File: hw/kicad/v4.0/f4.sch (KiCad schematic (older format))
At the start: 31 parts, among them P1 USB_OTG, U1 USBLC6-4SC6, U26 STM32F405VG, Y2 8M

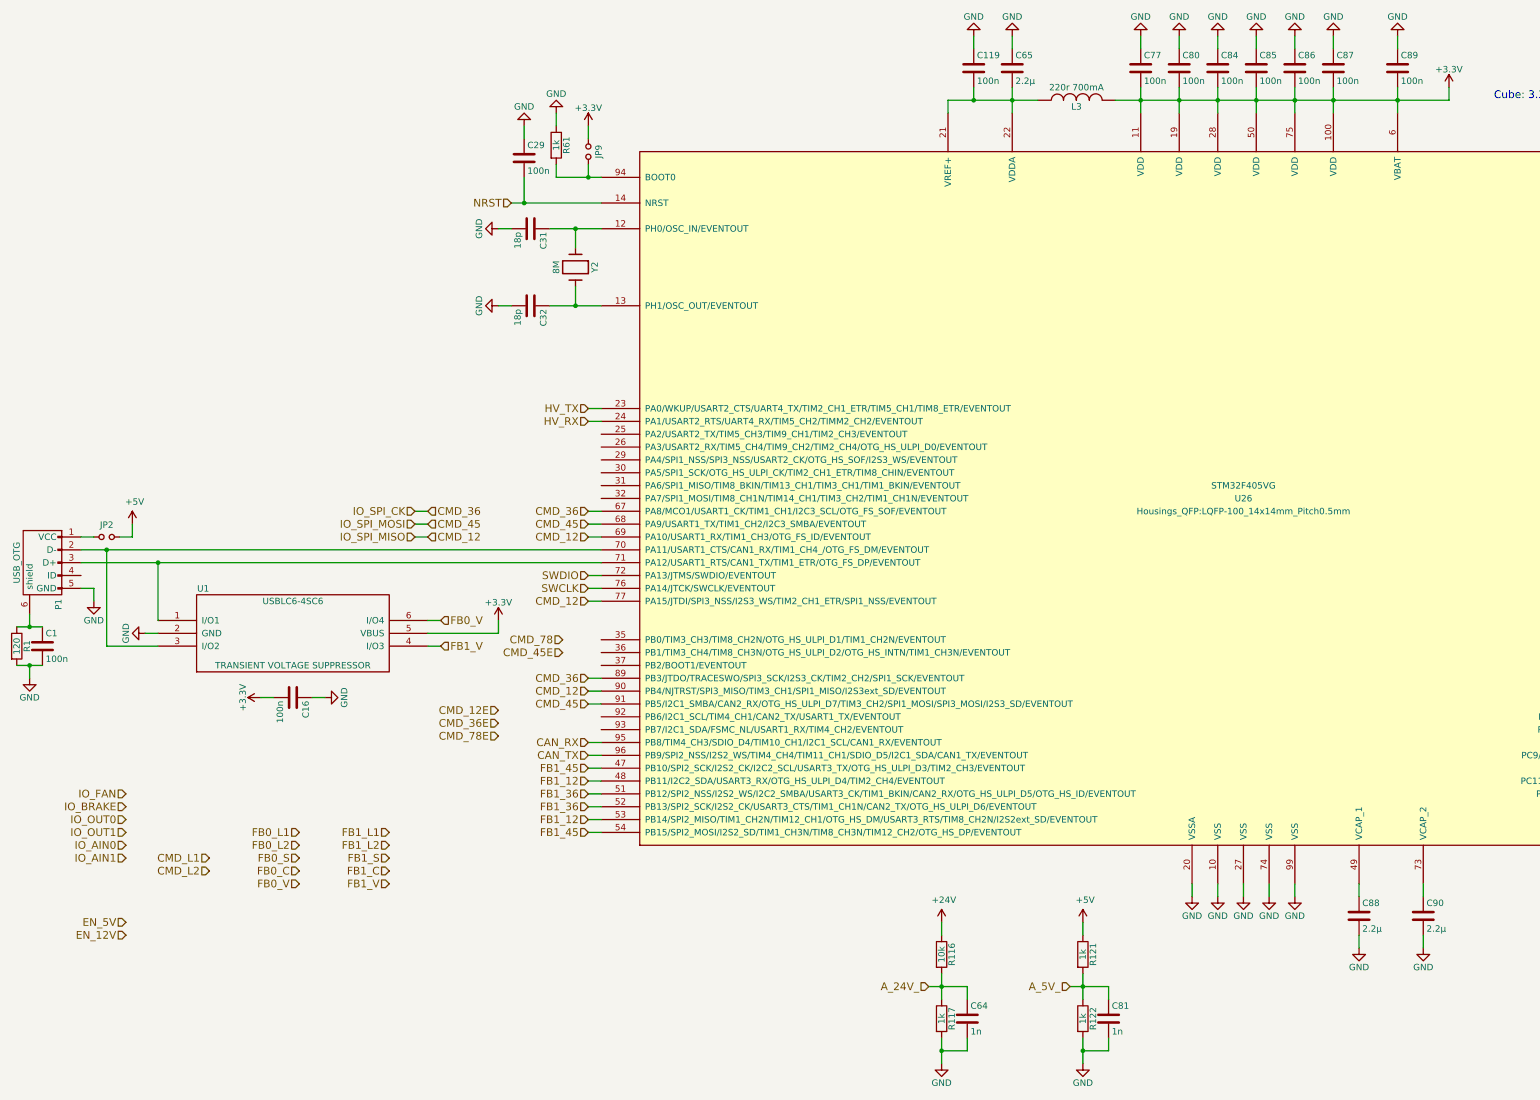
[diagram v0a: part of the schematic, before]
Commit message: v4.0
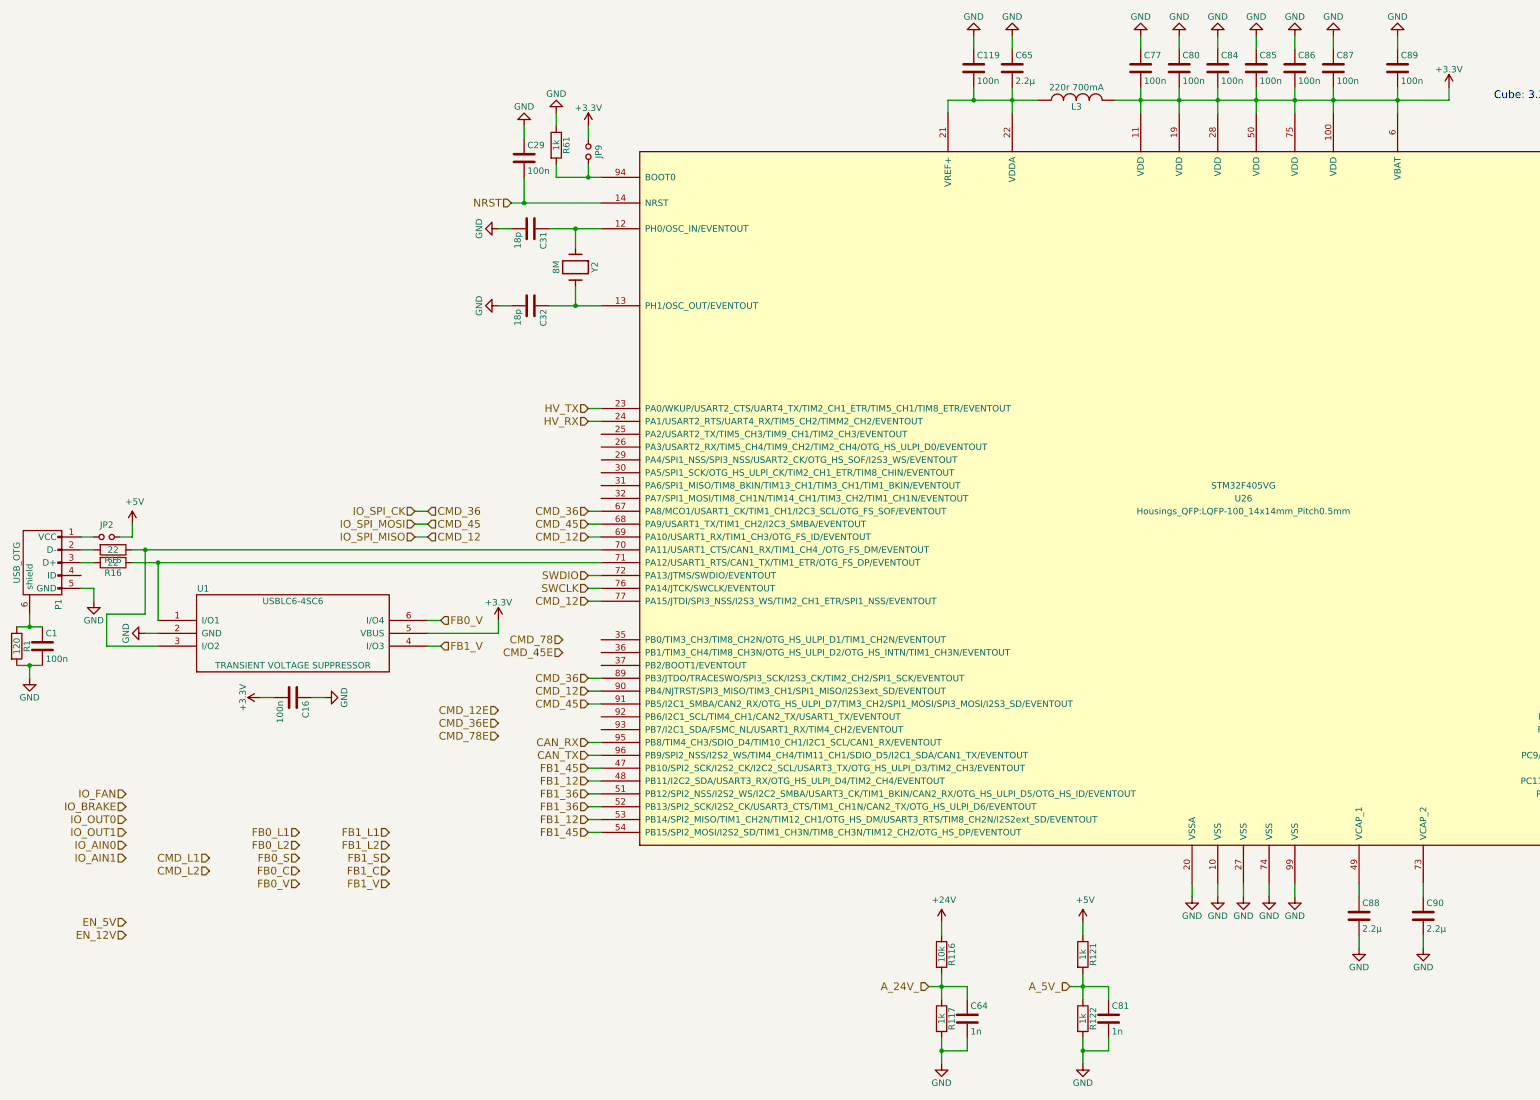
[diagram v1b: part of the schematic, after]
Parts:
- added R15, R16: 22, stmbl:R_0603, symbol R
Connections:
- net at U1.3 (I/O2), U26.70 (PA11/USART1_CTS/CAN1_RX/TIM1_CH4_/OTG_FS_DM/EVENTOUT): now also R15.1; no longer P1.2 (D-)
- net at U1.1 (I/O1), U26.71 (PA12/USART1_RTS/CAN1_TX/TIM1_ETR/OTG_FS_DP/EVENTOUT): now also R16.1; no longer P1.3 (D+)
- new net: P1.2 (D-), R15.2
- new net: P1.3 (D+), R16.2
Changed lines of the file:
@@
 $EndComp
 $Comp
-L GND #PWR0139
+L GND #PWR0140
 U 1 1 565FE0C3
 P 4400 4000
-F 0 "#PWR0139" H 4400 3750 50  0001 C CNN
+F 0 "#PWR0140" H 4400 3750 50  0001 C CNN
 F 1 "GND" H 4400 3850 50  0000 C CNN
 F 2 "" H 4400 4000 60  0000 C CNN
@@
 $EndComp
 $Comp
-L GND #PWR0140
+L GND #PWR0141
 U 1 1 565FE0E1
 P 4400 3400
-F 0 "#PWR0140" H 4400 3150 50  0001 C CNN
+F 0 "#PWR0141" H 4400 3150 50  0001 C CNN
 F 1 "GND" H 4400 3250 50  0000 C CNN
 F 2 "" H 4400 3400 60  0000 C CNN
@@
 $EndComp
 $Comp
-L GND #PWR0141
+L GND #PWR0142
 U 1 1 565FE268
 P 10600 8600
-F 0 "#PWR0141" H 10600 8350 50  0001 C CNN
+F 0 "#PWR0142" H 10600 8350 50  0001 C CNN
 F 1 "GND" H 10600 8450 50  0000 C CNN
 F 2 "" H 10600 8600 60  0000 C CNN
@@
 $EndComp
 $Comp
-L GND #PWR0142
+L GND #PWR0143
 U 1 1 565FE28C
 P 10400 8600
-F 0 "#PWR0142" H 10400 8350 50  0001 C CNN
+F 0 "#PWR0143" H 10400 8350 50  0001 C CNN
 F 1 "GND" H 10400 8450 50  0000 C CNN
 F 2 "" H 10400 8600 60  0000 C CNN
@@
 $EndComp
 $Comp
-L GND #PWR0143
+L GND #PWR0144
 U 1 1 565FE2A9
 P 10200 8600
-F 0 "#PWR0143" H 10200 8350 50  0001 C CNN
+F 0 "#PWR0144" H 10200 8350 50  0001 C CNN
 F 1 "GND" H 10200 8450 50  0000 C CNN
 F 2 "" H 10200 8600 60  0000 C CNN
@@
 $EndComp
 $Comp
-L GND #PWR0144
+L GND #PWR0145
 U 1 1 565FE2C6
 P 10000 8600
-F 0 "#PWR0144" H 10000 8350 50  0001 C CNN
+F 0 "#PWR0145" H 10000 8350 50  0001 C CNN
 F 1 "GND" H 10000 8450 50  0000 C CNN
 F 2 "" H 10000 8600 60  0000 C CNN
@@
 $EndComp
 $Comp
-L GND #PWR0145
+L GND #PWR0146
 U 1 1 565FE2E3
 P 9800 8600
-F 0 "#PWR0145" H 9800 8350 50  0001 C CNN
+F 0 "#PWR0146" H 9800 8350 50  0001 C CNN
 F 1 "GND" H 9800 8450 50  0000 C CNN
 F 2 "" H 9800 8600 60  0000 C CNN
@@
 $EndComp
 $Comp
-L GND #PWR0146
+L GND #PWR0147
 U 1 1 565FE300
 P 11100 9000
-F 0 "#PWR0146" H 11100 8750 50  0001 C CNN
+F 0 "#PWR0147" H 11100 8750 50  0001 C CNN
 F 1 "GND" H 11100 8850 50  0000 C CNN
 F 2 "" H 11100 9000 60  0000 C CNN
@@
 $EndComp
 $Comp
-L GND #PWR0147
+L GND #PWR0148
 U 1 1 565FE31D
 P 11600 9000
-F 0 "#PWR0147" H 11600 8750 50  0001 C CNN
+F 0 "#PWR0148" H 11600 8750 50  0001 C CNN
 F 1 "GND" H 11600 8850 50  0000 C CNN
 F 2 "" H 11600 9000 60  0000 C CNN
@@
 $EndComp
 $Comp
-L +3.3V #PWR0148
+L +3.3V #PWR0149
 U 1 1 565FEC9D
 P 11800 2300
-F 0 "#PWR0148" H 11800 2150 50  0001 C CNN
+F 0 "#PWR0149" H 11800 2150 50  0001 C CNN
 F 1 "+3.3V" H 11800 2440 50  0000 C CNN
 F 2 "" H 11800 2300 60  0000 C CNN
@@
 $EndComp
 $Comp
-L GND #PWR0149
+L GND #PWR0150
 U 1 1 565FECDB
 P 11400 1900
-F 0 "#PWR0149" H 11400 1650 50  0001 C CNN
+F 0 "#PWR0150" H 11400 1650 50  0001 C CNN
 F 1 "GND" H 11400 1750 50  0000 C CNN
 F 2 "" H 11400 1900 60  0000 C CNN
@@
 $EndComp
 $Comp
-L GND #PWR0150
+L GND #PWR0151
 U 1 1 565FED17
 P 10900 1900
-F 0 "#PWR0150" H 10900 1650 50  0001 C CNN
+F 0 "#PWR0151" H 10900 1650 50  0001 C CNN
 F 1 "GND" H 10900 1750 50  0000 C CNN
 F 2 "" H 10900 1900 60  0000 C CNN
@@
 $EndComp
 $Comp
-L GND #PWR0151
+L GND #PWR0152
 U 1 1 565FED4C
 P 10600 1900
-F 0 "#PWR0151" H 10600 1650 50  0001 C CNN
+F 0 "#PWR0152" H 10600 1650 50  0001 C CNN
 F 1 "GND" H 10600 1750 50  0000 C CNN
 F 2 "" H 10600 1900 60  0000 C CNN
@@
 $EndComp
 $Comp
-L GND #PWR0152
+L GND #PWR0153
 U 1 1 565FED81
 P 10300 1900
-F 0 "#PWR0152" H 10300 1650 50  0001 C CNN
+F 0 "#PWR0153" H 10300 1650 50  0001 C CNN
 F 1 "GND" H 10300 1750 50  0000 C CNN
 F 2 "" H 10300 1900 60  0000 C CNN
@@
 $EndComp
 $Comp
-L GND #PWR0153
+L GND #PWR0154
 U 1 1 565FEDB6
 P 10000 1900
-F 0 "#PWR0153" H 10000 1650 50  0001 C CNN
+F 0 "#PWR0154" H 10000 1650 50  0001 C CNN
 F 1 "GND" H 10000 1750 50  0000 C CNN
 F 2 "" H 10000 1900 60  0000 C CNN
@@
 $EndComp
 $Comp
-L GND #PWR0154
+L GND #PWR0155
 U 1 1 565FEDEB
 P 9700 1900
-F 0 "#PWR0154" H 9700 1650 50  0001 C CNN
+F 0 "#PWR0155" H 9700 1650 50  0001 C CNN
 F 1 "GND" H 9700 1750 50  0000 C CNN
 F 2 "" H 9700 1900 60  0000 C CNN
@@
 $EndComp
 $Comp
-L GND #PWR0155
+L GND #PWR0156
 U 1 1 565FEE20
 P 9400 1900
-F 0 "#PWR0155" H 9400 1650 50  0001 C CNN
+F 0 "#PWR0156" H 9400 1650 50  0001 C CNN
 F 1 "GND" H 9400 1750 50  0000 C CNN
 F 2 "" H 9400 1900 60  0000 C CNN
@@
 $EndComp
 $Comp
-L GND #PWR0156
+L GND #PWR0157
 U 1 1 565FF1AF
 P 8400 1900
-F 0 "#PWR0156" H 8400 1650 50  0001 C CNN
+F 0 "#PWR0157" H 8400 1650 50  0001 C CNN
 F 1 "GND" H 8400 1750 50  0000 C CNN
 F 2 "" H 8400 1900 60  0000 C CNN
@@
 	5100 4800 5200 4800
 Wire Wire Line
-	4800 3400 5000 3400
-Wire Wire Line
-	5000 3400 5200 3400
-Wire Wire Line
-	4800 4000 5000 4000
-Wire Wire Line
-	5000 4000 5200 4000
+	4800 3400 5200 3400
+Wire Wire Line
+	4800 4000 5200 4000
 Wire Wire Line
 	5000 3850 5000 4000
@@
 	9800 8500 9800 8600
 Wire Wire Line
-	11400 2300 11400 2400
-Wire Wire Line
-	11400 2400 11400 2500
-Wire Wire Line
-	10900 2300 10900 2400
-Wire Wire Line
-	10900 2400 10900 2500
-Wire Wire Line
-	10600 2300 10600 2400
-Wire Wire Line
-	10600 2400 10600 2500
-Wire Wire Line
-	10300 2300 10300 2400
-Wire Wire Line
-	10300 2400 10300 2500
-Wire Wire Line
-	10000 2300 10000 2400
-Wire Wire Line
-	10000 2400 10000 2500
-Wire Wire Line
-	9700 2300 9700 2400
-Wire Wire Line
-	9700 2400 9700 2500
-Wire Wire Line
-	9400 2300 9400 2400
-Wire Wire Line
-	9400 2400 9400 2500
-Wire Wire Line
-	9200 2400 9400 2400
-Wire Wire Line
-	9400 2400 9700 2400
-Wire Wire Line
-	9700 2400 10000 2400
-Wire Wire Line
-	10000 2400 10300 2400
-Wire Wire Line
-	10300 2400 10600 2400
-Wire Wire Line
-	10600 2400 10900 2400
-Wire Wire Line
-	10900 2400 11400 2400
-Wire Wire Line
-	11400 2400 11800 2400
+	11400 2300 11400 2500
+Wire Wire Line
+	10900 2300 10900 2500
+Wire Wire Line
+	10600 2300 10600 2500
+Wire Wire Line
+	10300 2300 10300 2500
+Wire Wire Line
+	10000 2300 10000 2500
+Wire Wire Line
+	9700 2300 9700 2500
+Wire Wire Line
+	9400 2300 9400 2500
+Wire Wire Line
+	9200 2400 11800 2400
 Connection ~ 9700 2400
 Connection ~ 9400 2400
@@
 	9400 2000 9400 1900
 Wire Wire Line
-	8400 2300 8400 2400
-Wire Wire Line
-	8400 2400 8400 2500
+	8400 2300 8400 2500
 Wire Wire Line
 	8400 2000 8400 1900
@@
 	7900 2500 7900 2400
 Wire Wire Line
-	7900 2400 8100 2400
-Wire Wire Line
-	8100 2400 8400 2400
-Wire Wire Line
-	8400 2400 8600 2400
+	7900 2400 8600 2400
 Connection ~ 8400 2400
 Wire Wire Line
@@
 	4600 2700 4600 2600
 Wire Wire Line
-	4500 3200 4600 3200
-Wire Wire Line
-	4600 3200 5200 3200
+	4500 3200 5200 3200
 Wire Wire Line
 	4600 3200 4600 3000
@@
 	15300 5400 15200 5400
 Wire Wire Line
-	650  6800 750  6800
-Wire Wire Line
-	750  6800 850  6800
+	650  6800 850  6800
 Wire Wire Line
 	750  6900 750  6800
@@
 	750  6400 750  6500
 Wire Wire Line
-	650  6500 750  6500
-Wire Wire Line
-	750  6500 850  6500
+	650  6500 850  6500
 Connection ~ 750  6500
 Wire Wire Line
@@
 	7850 8800 7850 8900
 Wire Wire Line
-	7850 9200 7850 9300
-Wire Wire Line
-	7850 9300 7850 9400
-Wire Wire Line
-	7850 9700 7850 9800
-Wire Wire Line
-	7850 9800 7850 9900
+	7850 9200 7850 9400
+Wire Wire Line
+	7850 9700 7850 9900
 Wire Wire Line
 	8950 8800 8950 8900
 Wire Wire Line
-	8950 9200 8950 9300
-Wire Wire Line
-	8950 9300 8950 9400
-Wire Wire Line
-	8950 9700 8950 9800
-Wire Wire Line
-	8950 9800 8950 9900
-Wire Wire Line
-	8850 9300 8950 9300
-Wire Wire Line
-	8950 9300 9150 9300
+	8950 9200 8950 9400
+Wire Wire Line
+	8950 9700 8950 9900
+Wire Wire Line
+	8850 9300 9150 9300
 Connection ~ 8950 9300
 Wire Wire Line
-	7750 9300 7850 9300
-Wire Wire Line
-	7850 9300 8050 9300
+	7750 9300 8050 9300
 Connection ~ 7850 9300
 Wire Wire Line
@@
 	4850 2900 4850 3000
 Wire Wire Line
-	4850 3000 5100 3000
-Wire Wire Line
-	5100 3000 5200 3000
+	4850 3000 5200 3000
 Wire Wire Line
 	5100 2900 5100 3000
@@
 	5100 2600 5100 2700
 Wire Wire Line
-	1150 6000 1750 6000
-Wire Wire Line
-	1750 6000 5200 6000
-Wire Wire Line
-	1150 5900 1350 5900
-Wire Wire Line
-	1350 5900 5200 5900
+	1550 6000 5200 6000
 Wire Wire Line
 	1750 6450 1750 6000
 Connection ~ 1750 6000
-Wire Wire Line
-	1750 6650 1350 6650
-Wire Wire Line
-	1350 6650 1350 5900
-Connection ~ 1350 5900
 Wire Wire Line
 	1650 6550 1750 6550
@@
 Wire Wire Line
 	15300 4400 15200 4400
+$Comp
+L R R16
+U 1 1 57F851F7
+P 1400 6000
+F 0 "R16" V 1480 6000 50  0000 C CNN
+F 1 "22" V 1400 6000 50  0000 C CNN
+F 2 "stmbl:R_0603" V 1330 6000 30  0001 C CNN
+F 3 "" H 1400 6000 30  0000 C CNN
+	1    1400 6000
+	0    1    1    0
+$EndComp
+Wire Wire Line
+	1250 6000 1150 6000
+$Comp
+L R R15
+U 1 1 57F85A1B
+P 1400 5900
+F 0 "R15" V 1480 5900 50  0000 C CNN
+F 1 "22" V 1400 5900 50  0000 C CNN
+F 2 "stmbl:R_0603" V 1330 5900 30  0001 C CNN
+F 3 "" H 1400 5900 30  0000 C CNN
+	1    1400 5900
+	0    1    1    0
+$EndComp
+Wire Wire Line
+	1750 6650 1350 6650
+Wire Wire Line
+	1350 6650 1350 6400
+Wire Wire Line
+	1350 6400 1650 6400
+Wire Wire Line
+	1650 6400 1650 5900
+Connection ~ 1650 5900
+Wire Wire Line
+	1550 5900 5200 5900
+Wire Wire Line
+	1250 5900 1150 5900
 $EndSCHEMATC
